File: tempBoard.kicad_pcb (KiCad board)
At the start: 2 copper layers, 32.3 x 51.6 mm, 11 parts, among them J1 OLED_128X64_1.3_I2C, U1 SHTC3, U2 XIAO-RP2040-DIP

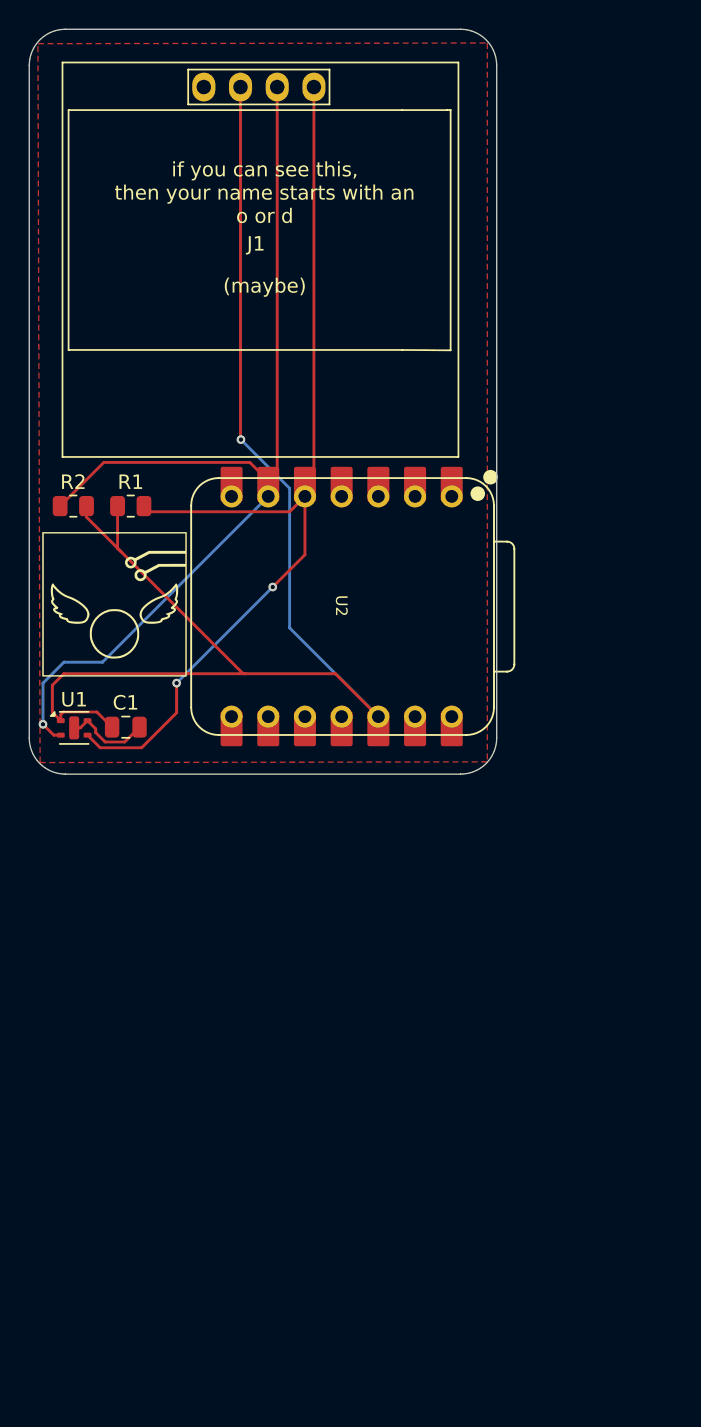
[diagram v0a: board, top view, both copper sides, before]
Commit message: remake pcb
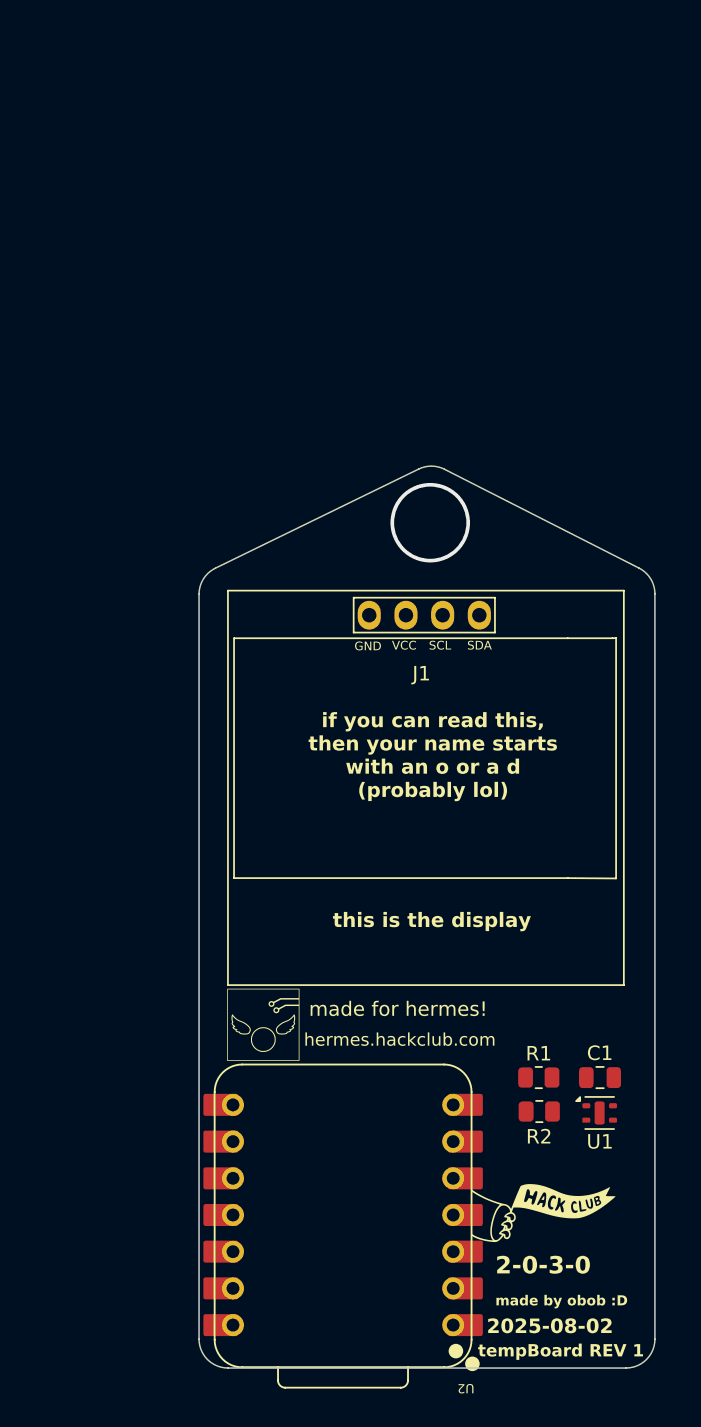
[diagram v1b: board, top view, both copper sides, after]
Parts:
- removed the G*** at (144.7, 59.1)
- removed the G*** at (156.4, 30.8)
- removed the G*** at (166.1, 23.8)
- removed the G*** at (162.8, 42.8)
- removed the G*** at (146.8, 42.5)
- added G***: LOGO, LOGO, F.Cu at (154.9, 88.2)
- added G***: LOGO, LOGO, F.Cu at (174.3, 101.2)
- added G***: LOGO, LOGO, B.Cu at (166.2, 70.8)
- U1: footprint Sensor_Humidity:Sensirion_DFN-4-1EP_2x2mm_P1mm_EP0.7x1.6mm -> general:Sensirion_DFN-4-1EP_2x2mm_P1mm_EP0.7x1.6mm
- moved R2 52.9 mm to (174.1, 94.2)
- moved R1 48.6 mm to (174.0, 91.9)
- moved U1 45.1 mm to (178.2, 94.3)
- moved U2 42.1 mm to (160.5, 101.4), turned to 180 degrees
- moved C1 40.8 mm to (178.2, 91.9)
- moved J1 38.3 mm to (165.9, 70.5)
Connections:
- U1 pad 5: GND -> unconnected-(U1-NC-Pad5)
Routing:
- net +3V3: track 98.6 -> 0.00 mm, vias 1 -> 0
- net SCL: track 70.3 -> 0.00 mm, vias 1 -> 0
- net SDA: track 66.5 -> 0.00 mm, vias 2 -> 0
- net GND: track 5.92 -> 0.00 mm
- net (no net): vias 0 -> 1
- removed copper zone on F.Cu, net GND
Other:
- board size 32.3 x 51.6 mm -> 31.6 x 62.4 mm
- board text added: "2-0-3-0"
- board text added: "2025-08-02"
- board text added: "GND"
- board text added: "ISO 8601 ftw!!!"
- board text added: "SCL"
- board text added: "SDA"
- board text added: "VCC"
- board text added: "hermes.hackclub.com"
- board text added: "if you can read this, then your name starts with an o or a d (probably lol)"
- board text added: "made by obob :D"
- board text added: "made for hermes!"
- board text added: "self-promotion (pls scan)"
- board text added: "tempBoard REV 1"
- board text added: "the thing with a hole is the sensor itself"
- board text added: "this is a decoupling capactitor, it filters out noise"
- board text added: "this is the display"
- board text added: "this is the microcontroller, its like the brain of this board"
- board text added: "you can use this on a key ring!"
- board text removed: "hermes!"
- board text removed: "if you can see this, then your name starts with an o or d (maybe)"
- board text removed: "more specifically, the SHTC3"
- board text removed: "this is the microcontroller, the brains of this device"
- board text removed: "this is the temperature and humidity sensor"
